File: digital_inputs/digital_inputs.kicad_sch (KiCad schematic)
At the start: 112 parts, among them J1 6437288-2, J10 Conn_01x01, J11 Conn_01x01, J12 Conn_01x01, J13 Conn_01x01, J14 Conn_01x01, J15 Conn_01x01, J16 Conn_01x01, J17 Conn_01x01, J19 6437288-3, J3 Conn_01x08, J4 Conn_01x01, J5 Conn_01x02, J6 Conn_01x04, J7 Conn_01x04, J8 Conn_01x04, J9 Conn_01x04, Q1 AO3400A, Q2 AO3400A, Q3 AO3400A, Q4 AO3400A, Q5 AO3400A, Q6 AO3400A, Q7 AO3400A, Q8 AO3400A, U1 OPA4192IPW, U10 ULN2003A, U11 NUCLEO-F429ZI, U12 TJA1051T-3, U2 CD4067BM96, U3 CD4067BM96, U4 CD4067BM96, U5 CD4067BM96, U6 CD4067BM96, U7 CD4067BM96, U8 TC4427, U9 TC4427

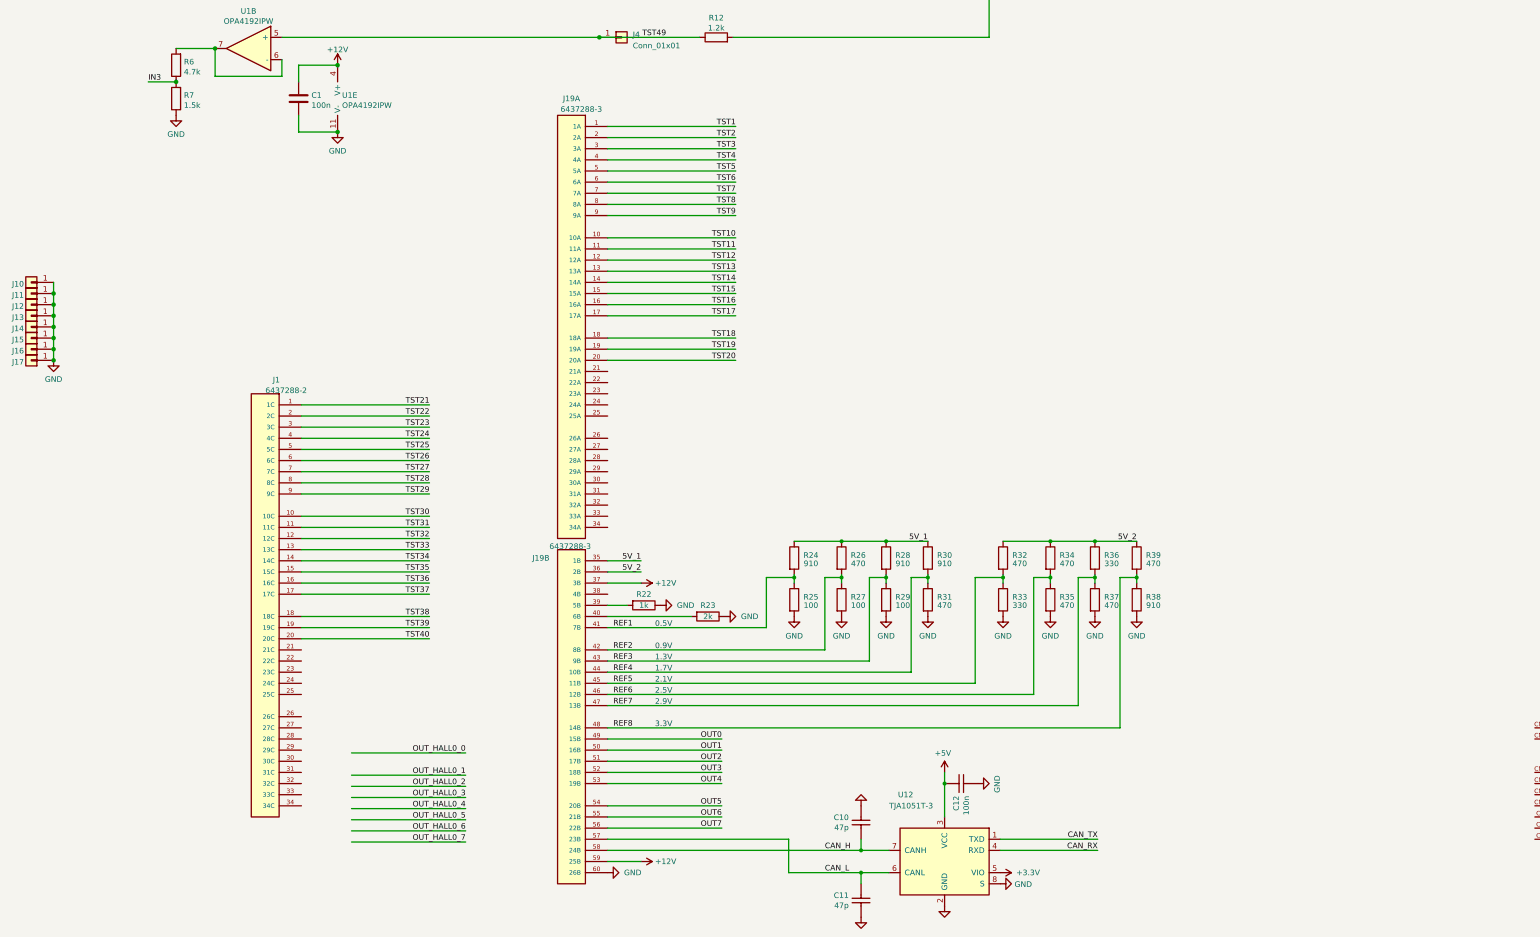
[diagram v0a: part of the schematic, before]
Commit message: #16 #17
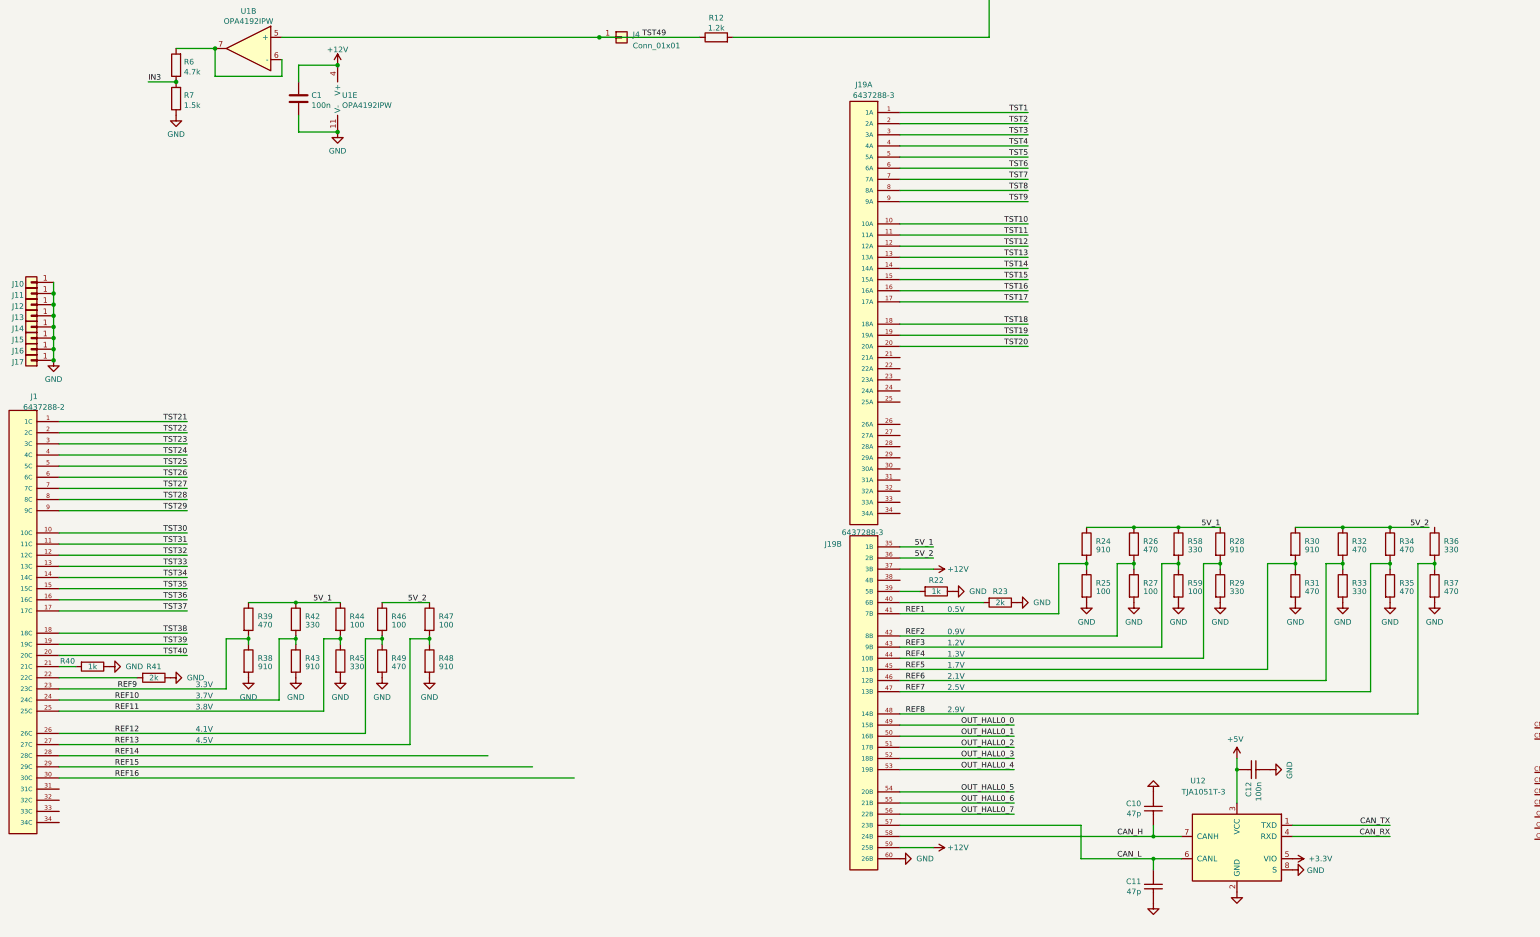
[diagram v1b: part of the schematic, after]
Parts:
- added R40: 1k, Resistor_SMD:R_0603_1608Metric, symbol Device:R
- added R41: 2k, Resistor_SMD:R_0603_1608Metric, symbol Device:R
- added R42, R45, R58: 330, Resistor_SMD:R_0603_1608Metric, symbol Device:R
- added R43, R48: 910, Resistor_SMD:R_0603_1608Metric, symbol Device:R
- added R44, R46, R47, R59: 100, Resistor_SMD:R_0603_1608Metric, symbol Device:R
- added R49: 470, Resistor_SMD:R_0603_1608Metric, symbol Device:R
- R29: value 100 -> 330
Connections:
- net OUT4 is gone; now on net OUT_HALL0_4: J19.53 (19B)
- net OUT5 is gone; now on net OUT_HALL0_5: J19.54 (20B)
- net OUT6 is gone; now on net OUT_HALL0_6: J19.55 (21B)
- net OUT7 is gone; now on net OUT_HALL0_7: J19.56 (22B)
- net 5V_1: now also R39.1, R42.1, R44.1, R58.1; no longer R30.1
- net 5V_2: now also R30.1, R46.1, R47.1; no longer R36.1, R39.1
- net GND: now also R40.1, R41.1, R43.2, R45.2, R48.2, R49.2, R59.2
- net OUT0: no longer J19.49 (15B)
- net OUT1: no longer J19.50 (16B)
- net OUT2: no longer J19.51 (17B)
- net OUT3: no longer J19.52 (18B)
- net OUT_HALL0_0: now also J19.49 (15B)
- net OUT_HALL0_1: now also J19.50 (16B)
- net OUT_HALL0_2: now also J19.51 (17B)
- net OUT_HALL0_3: now also J19.52 (18B)
- net REF3: now also R58.2, R59.1; no longer R28.2, R29.1
- net REF4: now also R28.2, R29.1; no longer R30.2, R31.1
- net REF5: now also R30.2, R31.1; no longer R32.2, R33.1
- net REF6: now also R32.2, R33.1; no longer R34.2, R35.1
- net REF7: now also R34.2, R35.1; no longer R36.2, R37.1
- net REF8: now also R36.2, R37.1; no longer R38.1, R39.2
- net at J1.21 (21C): now also R40.2
- net at J1.22 (22C): now also R41.2
- net REF9: now reaches J1.23 (23C)
- net REF9: now also R38.1, R39.2
- net REF10: now reaches J1.24 (24C)
- net REF10: now also R42.2, R43.1
- net REF11: now reaches J1.25 (25C)
- net REF11: now also R44.2, R45.1
- net REF12: now reaches J1.26 (26C)
- net REF12: now also R46.2, R49.1
- net REF13: now reaches J1.27 (27C)
- net REF13: now also R47.2, R48.1
- net REF14: now reaches J1.28 (28C)
- net REF15: now reaches J1.29 (29C)
- net REF16: now reaches J1.30 (30C)
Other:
- note added: "1.2V"
- note added: "3.7V"
- note added: "3.8V"
- note added: "4.1V"
- note added: "4.5V"
- moved on the sheet: C10, C11, C12, J1, J19A, J19B, R22, R23, R24, R25, R26, R27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
